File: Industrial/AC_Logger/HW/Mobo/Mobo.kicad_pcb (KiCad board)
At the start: 2 copper layers, 78.7 x 43.2 mm, 5 parts

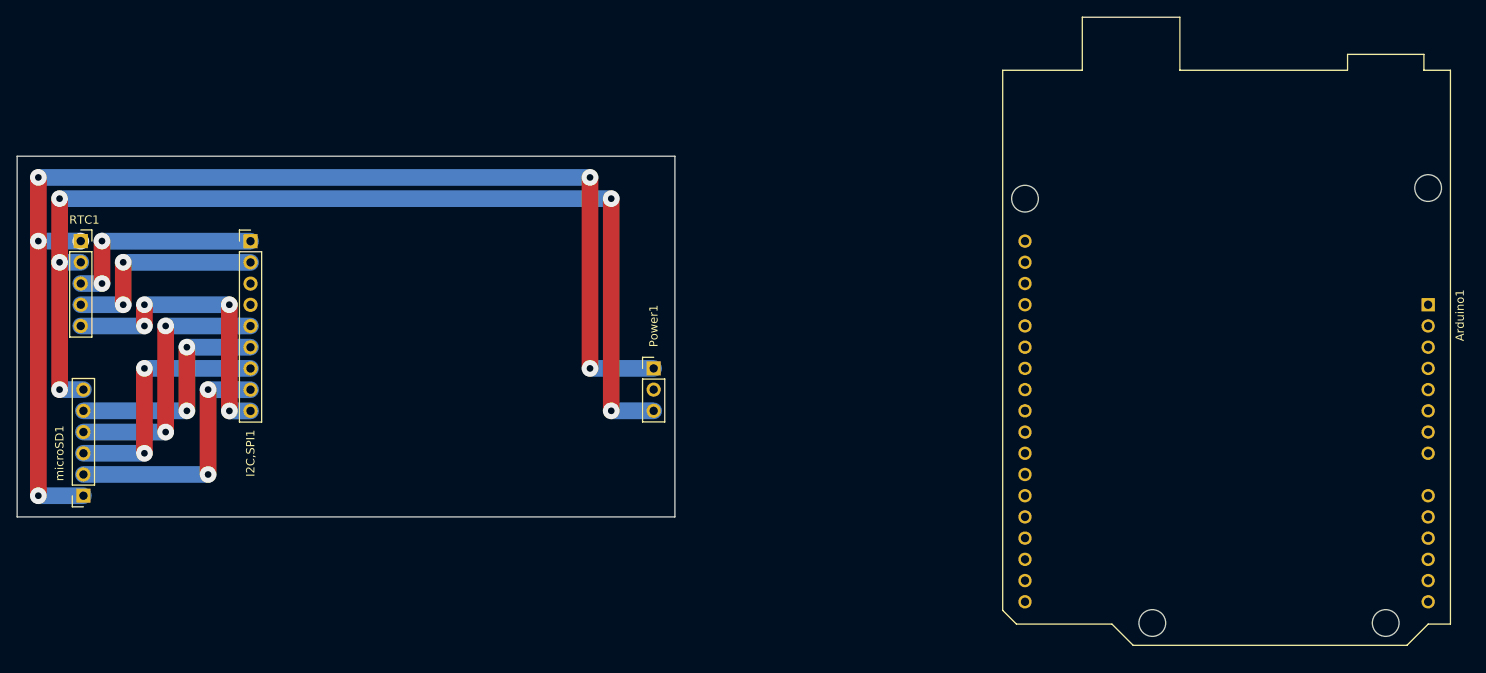
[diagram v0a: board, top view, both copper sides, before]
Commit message: Last last edit to pcb
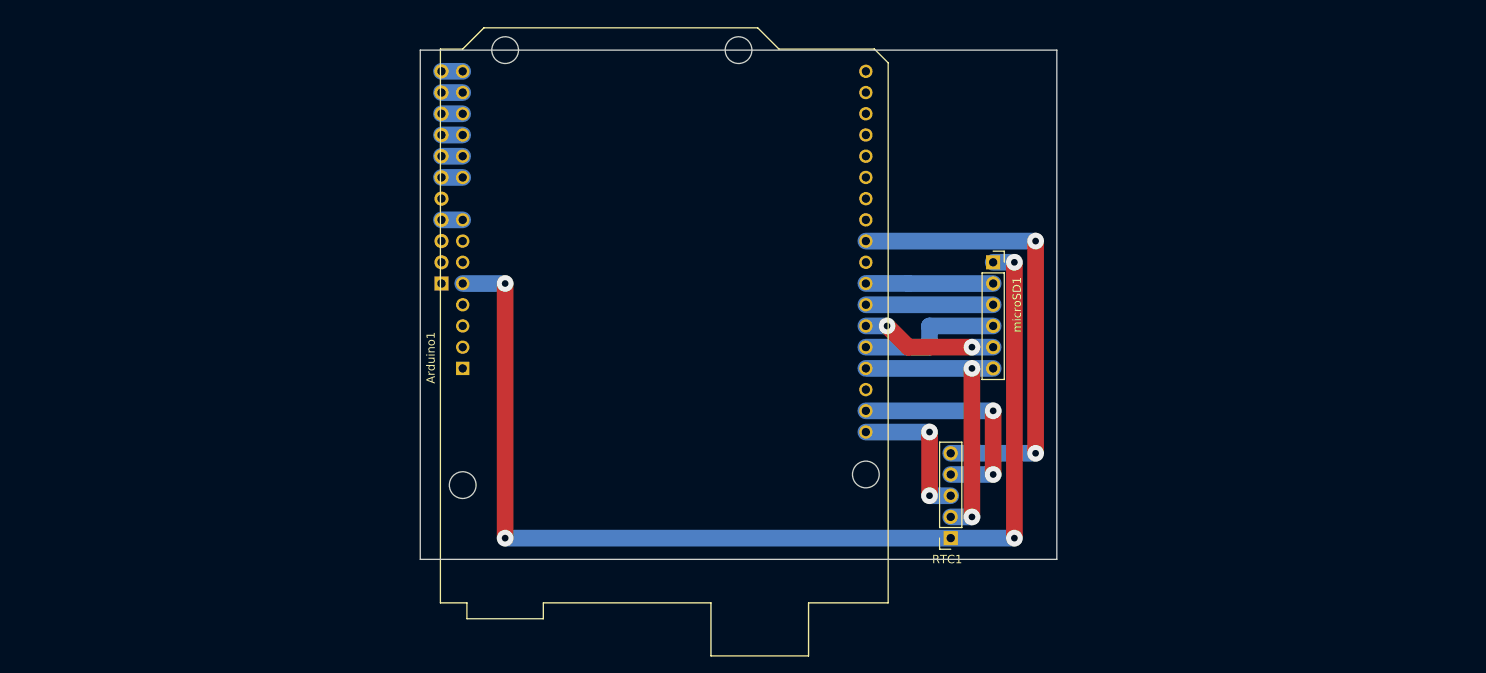
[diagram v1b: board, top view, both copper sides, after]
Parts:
- removed I2C,SPI1: Conn_01x09_Male, Connector_PinHeader_2.54mm:PinHeader_1x09_P2.54mm_Vertical
- removed Power1: Conn_01x03_Male, Connector_PinHeader_2.54mm:PinHeader_1x03_P2.54mm_Vertical
- added J1: Conn_01x11_Female, Connector_PinSocket_2.54mm:PinSocket_1x11_P2.54mm_Vertical, B.Cu at (114.3, 94.0)
- moved Arduino1 115.8 mm to (116.8, 104.1), turned to 90 degrees
- moved microSD1 112.4 mm to (180.3, 91.4), turned to 0 degrees
- moved RTC1 110.0 mm to (175.3, 124.5), turned to 180 degrees
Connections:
- Arduino1 pad 10: unconnected-(Arduino1-Pad10) -> /A1
- Arduino1 pad 11: unconnected-(Arduino1-Pad11) -> /A2
- Arduino1 pad 12: unconnected-(Arduino1-Pad12) -> /A3
- Arduino1 pad 13: unconnected-(Arduino1-Pad13) -> /A4
- Arduino1 pad 14: unconnected-(Arduino1-Pad14) -> /A5
- Arduino1 pad 23: unconnected-(Arduino1-Pad23) -> /RTC RST
- Arduino1 pad 24: /RTC RST -> unconnected-(Arduino1-Pad24)
- Arduino1 pad 29: unconnected-(Arduino1-Pad29) -> GND
- Arduino1 pad 4: /3V3 -> unconnected-(Arduino1-Pad4)
- Arduino1 pad 5: /5V -> +5V
- Arduino1 pad 6: /GND -> GND
- Arduino1 pad 7: unconnected-(Arduino1-Pad7) -> GND
- Arduino1 pad 8: unconnected-(Arduino1-Pad8) -> /VIN
- Arduino1 pad 9: unconnected-(Arduino1-Pad9) -> /A0
- RTC1 pad 1: /3V3 -> +5V
- RTC1 pad 2: /GND -> GND
- microSD1 pad 1: /3V3 -> +5V
- microSD1 pad 6: /GND -> GND
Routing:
- net /3V3: track 145.1 -> 0.00 mm, vias 6 -> 0
- net +5V: track 0.00 -> 132.1 mm, vias 0 -> 4
- net /GND: track 124.8 -> 0.00 mm, vias 5 -> 0
- net GND: track 0.00 -> 35.6 mm, vias 0 -> 2
- net /RTC RST: track 35.6 -> 55.9 mm, vias 4 -> 2
- net /SS: track 30.2 -> 15.2 mm, vias 2 -> 0
- net /SCK: track 32.7 -> 17.8 mm, vias 2 -> 0
- net /MOSI: track 30.2 -> 15.2 mm, vias 2 -> 0
- net /MISO: track 27.6 -> 16.3 mm
- net /SCL: track 25.4 -> 17.8 mm
- net /VIN: track 0.00 -> 2.54 mm
- net /A5: track 0.00 -> 2.54 mm
- net /A4: track 0.00 -> 2.54 mm
- net /A3: track 0.00 -> 2.54 mm
- net /A2: track 0.00 -> 2.54 mm
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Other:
- board size 78.7 x 43.2 mm -> 76.2 x 61 mm
